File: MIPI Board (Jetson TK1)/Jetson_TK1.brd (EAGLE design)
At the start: 50.5 x 57.1 mm, 19 parts, among them IC2 TPS77001, IC3 LM340MP-05, J1 MYLIBRARY_Q1S02B, U1 J3A2

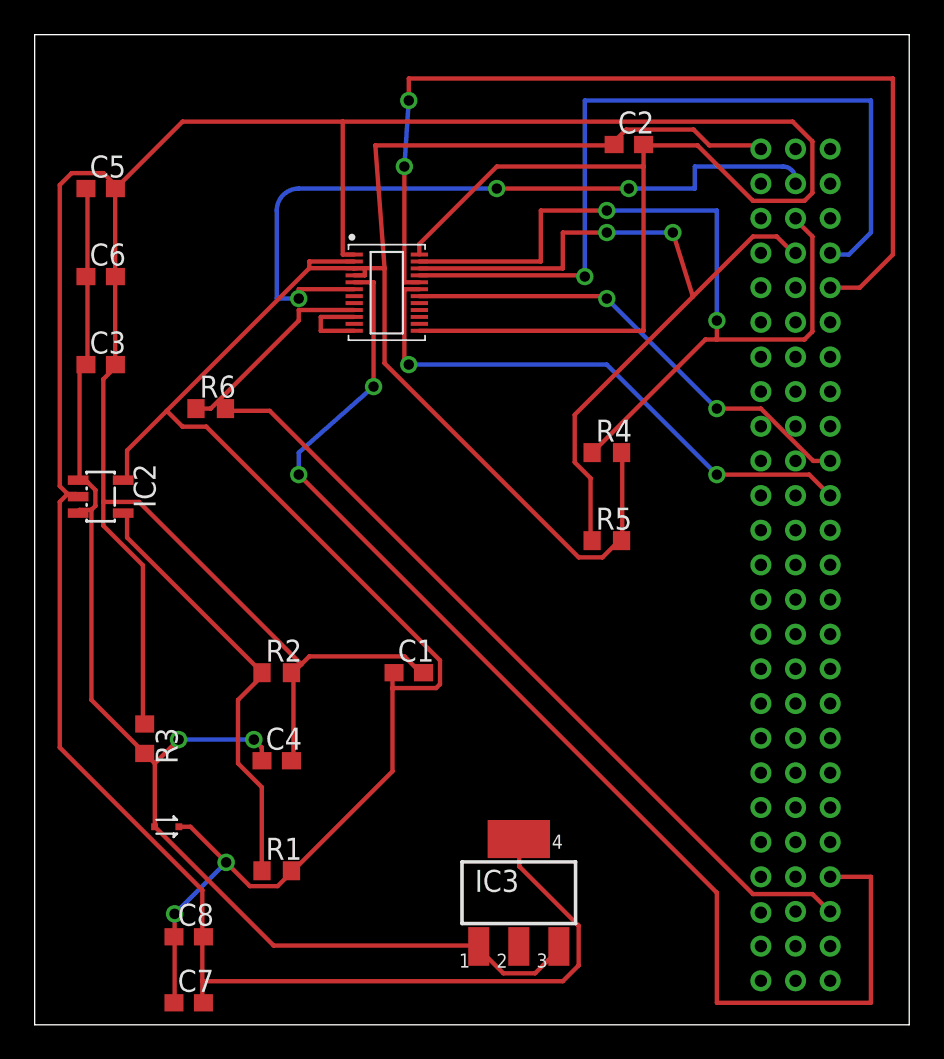
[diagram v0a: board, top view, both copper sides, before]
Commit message: Updated BRD
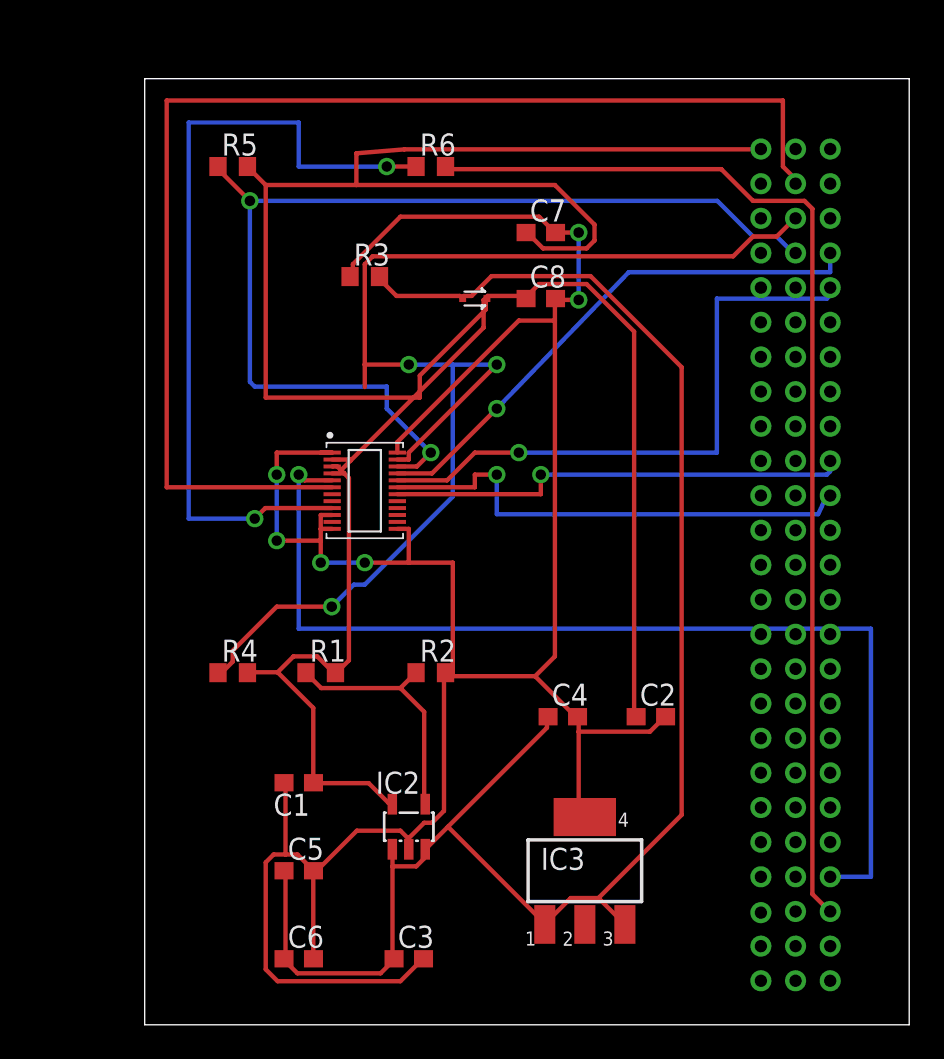
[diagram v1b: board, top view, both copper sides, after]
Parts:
- moved C7 48.9 mm to (78.7, 45.7)
- moved C8 42.1 mm to (78.7, 41.9)
- moved C5 41.0 mm to (64.8, 8.89)
- moved C6 41.0 mm to (64.8, 3.81)
- moved C3 38.6 mm to (71.1, 3.81)
- moved D1 35.3 mm to (74.9, 41.9)
- moved C2 33.0 mm to (85.1, 17.8)
- moved R5 30.5 mm to (61.0, 49.5)
- moved R3 29.5 mm to (68.6, 43.2), turned to 0 degrees
- moved IC2 26.1 mm to (71.1, 11.4), turned to 0 degrees
- moved R4 25.0 mm to (61.0, 20.3)
- moved R6 18.9 mm to (72.4, 49.5)
- moved C4 16.7 mm to (80.0, 17.8)
- moved R1 11.7 mm to (66.0, 20.3)
- moved J1 11.5 mm to (68.6, 33.0)
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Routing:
- net PE: track 256.2 -> 154.7 mm, vias 0 -> 6
- net N$9: track 11.8 -> 47.1 mm, vias 0 -> 2
- net N$11: track 42.4 -> 72.5 mm, vias 3 -> 0
- net N$4: track 50.1 -> 74.7 mm, vias 2 -> 3
- net VCC: track 75.7 -> 99.0 mm, vias 2 -> 0
- net N$6: track 55.1 -> 35.1 mm, vias 2 -> 1
- net VDD: track 142.3 -> 159.5 mm, vias 2 -> 0
- net N$3: track 47.2 -> 31.0 mm
- net N$10: track 47.0 -> 63.2 mm
- net N$5: track 45.6 -> 61.0 mm
- net N$12: track 73.2 -> 60.6 mm, vias 2 -> 1
- net N$2: track 25.2 -> 14.4 mm
- net N$7: track 32.8 -> 28.7 mm, vias 2 -> 1
- net N$8: track 27.6 -> 26.8 mm, vias 2 -> 1
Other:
- board size 50.5 x 57.1 mm -> 44.1 x 54.6 mm
